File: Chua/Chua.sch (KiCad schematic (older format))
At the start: 19 parts, among them P1 CONN_01X03, U1 TL082, U2 TL082

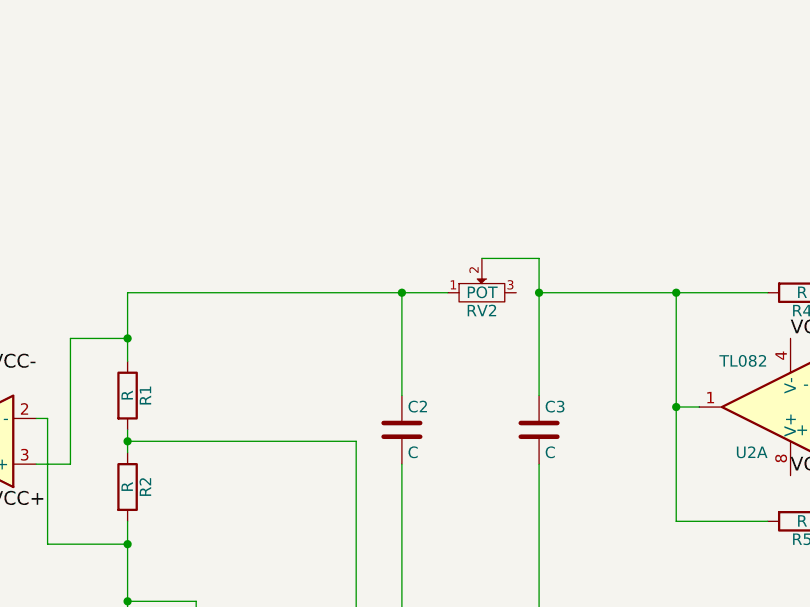
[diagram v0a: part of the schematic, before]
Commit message: adding output to chua
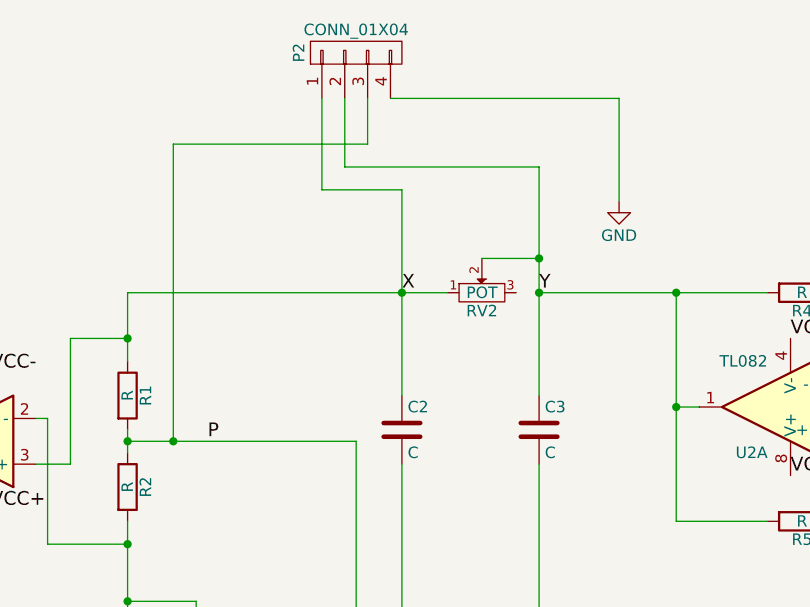
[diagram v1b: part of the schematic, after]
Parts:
- added P2: CONN_01X04, Pin_Headers:Pin_Header_Straight_1x04_Pitch2.54mm, symbol CONN_01X04
- P1: footprint (none) -> Pin_Headers:Pin_Header_Straight_1x03_Pitch2.54mm
- RV1, RV2: footprint (none) -> DM_Custom:DM_POT_296
- U1, U2: footprint (none) -> DM_Custom:DM_TSSOP8
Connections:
- net GND: now also P2.4 (P4)
- net Y: now reaches C3.1, R4.2, R5.2, RV2.2, U2.1
- net Y: now also P2.2 (P2)
- net X: now reaches C2.1, R1.1, RV2.1, U1.3 (+)
- net X: now also P2.1 (P1)
- net P: now reaches R1.2, R2.1, U1.7
- net P: now also P2.3 (P3)
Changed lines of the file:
@@
 F 0 "U2" H 9150 2550 50  0000 L CNN
 F 1 "TL082" H 9150 2150 50  0000 L CNN
-F 2 "" H 9150 2350 50  0001 C CNN
+F 2 "DM_Custom:DM_TSSOP8" H 9150 2350 50  0001 C CNN
 F 3 "" H 9150 2350 50  0000 C CNN
 	2    9150 2350
@@
 F 0 "U2" H 7900 2550 50  0000 L CNN
 F 1 "TL082" H 7900 2150 50  0000 L CNN
-F 2 "" H 7900 2350 50  0001 C CNN
+F 2 "DM_Custom:DM_TSSOP8" H 7900 2350 50  0001 C CNN
 F 3 "" H 7900 2350 50  0000 C CNN
 	1    7900 2350
@@
 F 0 "U1" H 4400 2700 50  0000 L CNN
 F 1 "TL082" H 4400 2300 50  0000 L CNN
-F 2 "" H 4400 2500 50  0001 C CNN
+F 2 "DM_Custom:DM_TSSOP8" H 4400 2500 50  0001 C CNN
 F 3 "" H 4400 2500 50  0000 C CNN
 	1    4400 2500
@@
 F 0 "U1" H 5800 3850 50  0000 L CNN
 F 1 "TL082" H 5800 3450 50  0000 L CNN
-F 2 "" H 5800 3650 50  0001 C CNN
+F 2 "DM_Custom:DM_TSSOP8" H 5800 3650 50  0001 C CNN
 F 3 "" H 5800 3650 50  0000 C CNN
 	2    5800 3650
@@
 F 0 "RV1" H 5650 4670 50  0000 C CNN
 F 1 "POT" H 5650 4750 50  0000 C CNN
-F 2 "" H 5650 4750 50  0001 C CNN
+F 2 "DM_Custom:DM_POT_296" H 5650 4750 50  0001 C CNN
 F 3 "" H 5650 4750 50  0000 C CNN
 	1    5650 4750
@@
 F 0 "RV2" H 6650 1770 50  0000 C CNN
 F 1 "POT" H 6650 1850 50  0000 C CNN
-F 2 "" H 6650 1850 50  0001 C CNN
+F 2 "DM_Custom:DM_POT_296" H 6650 1850 50  0001 C CNN
 F 3 "" H 6650 1850 50  0000 C CNN
 	1    6650 1850
@@
 Connection ~ 7500 1850
 Wire Wire Line
-	6900 1700 6900 2300
+	6900 1300 6900 2300
 Connection ~ 6900 1850
 Wire Wire Line
 	5100 1850 6500 1850
 Wire Wire Line
-	6300 1850 6300 2300
+	6300 1400 6300 2300
 Wire Wire Line
 	5100 1850 5100 2150
@@
 F 0 "P1" H 2700 3400 50  0000 C CNN
 F 1 "CONN_01X03" V 2800 3200 50  0000 C CNN
-F 2 "" H 2700 3200 50  0001 C CNN
+F 2 "Pin_Headers:Pin_Header_Straight_1x03_Pitch2.54mm" H 2700 3200 50  0001 C CNN
 F 3 "" H 2700 3200 50  0000 C CNN
 	1    2700 3200
@@
 	3300 3600 3300 3950
 Connection ~ 3300 3950
+Text Label 6300 1850 0    60   ~ 0
+X
+Text Label 6900 1850 0    60   ~ 0
+Y
+Text Label 5450 2500 0    60   ~ 0
+P
+Connection ~ 5300 2500
+$Comp
+L CONN_01X04 P2
+U 1 1 59307B52
+P 6100 800
+F 0 "P2" H 6100 1050 50  0000 C CNN
+F 1 "CONN_01X04" V 6200 800 50  0000 C CNN
+F 2 "Pin_Headers:Pin_Header_Straight_1x04_Pitch2.54mm" H 6100 800 50  0001 C CNN
+F 3 "" H 6100 800 50  0000 C CNN
+	1    6100 800
+	0    -1   -1   0
+$EndComp
+$Comp
+L GND #PWR03
+U 1 1 59306F49
+P 7250 1450
+F 0 "#PWR03" H 7250 1200 50  0001 C CNN
+F 1 "GND" H 7250 1300 50  0000 C CNN
+F 2 "" H 7250 1450 50  0000 C CNN
+F 3 "" H 7250 1450 50  0000 C CNN
+	1    7250 1450
+	1    0    0    -1
+$EndComp
+Wire Wire Line
+	6250 1000 7250 1000
+Wire Wire Line
+	7250 1000 7250 1450
+Wire Wire Line
+	6900 1300 6050 1300
+Wire Wire Line
+	6050 1300 6050 1000
+Connection ~ 6900 1700
+Wire Wire Line
+	6300 1400 5950 1400
+Wire Wire Line
+	5950 1400 5950 1000
+Wire Wire Line
+	5300 2500 5300 1200
+Wire Wire Line
+	5300 1200 6150 1200
+Wire Wire Line
+	6150 1200 6150 1000
 $EndSCHEMATC
